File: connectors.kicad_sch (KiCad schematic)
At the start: 31 parts, among them J1 Conn_01x02, J2 USB_B_Micro, J3 Conn_01x04, J4 Conn_01x04, J5 Conn_01x04, J6 Conn_01x04, J7 Conn_01x04, J8 Conn_01x04, J9 Conn_02x05_Odd_Even, U4 USBLC6-2SC6

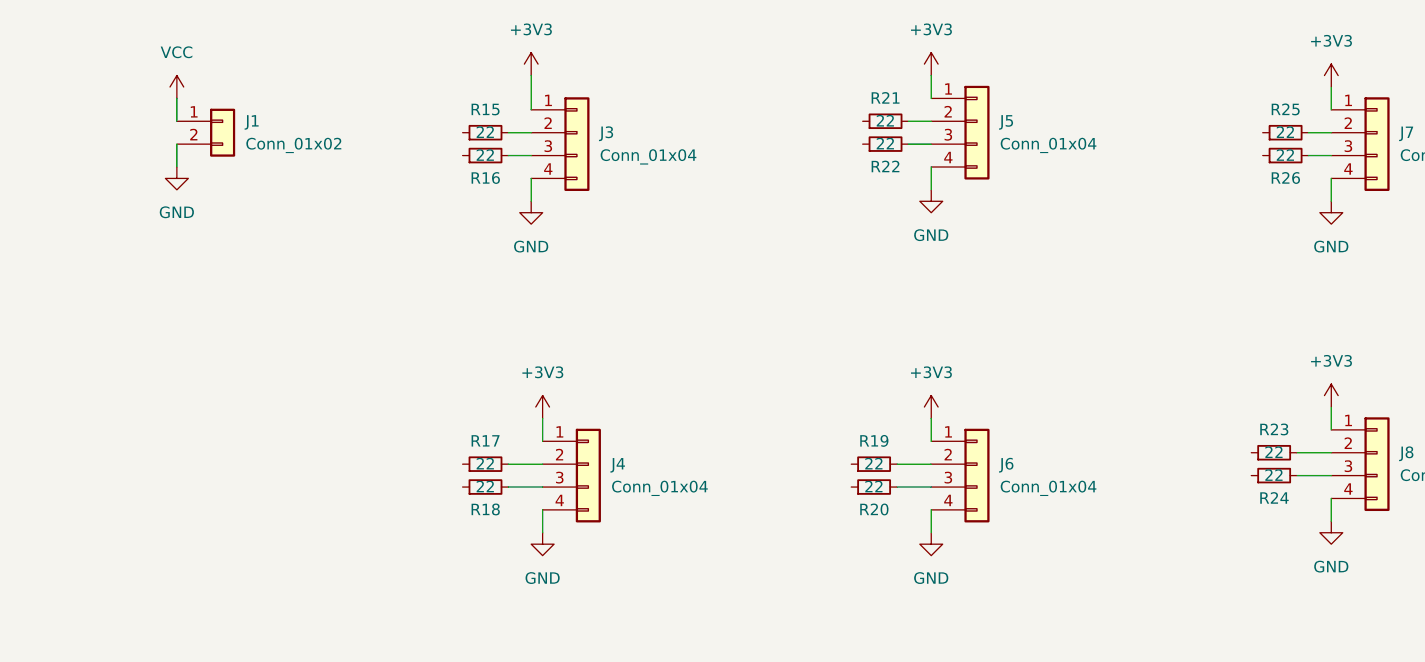
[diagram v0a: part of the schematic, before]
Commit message: updated schematic
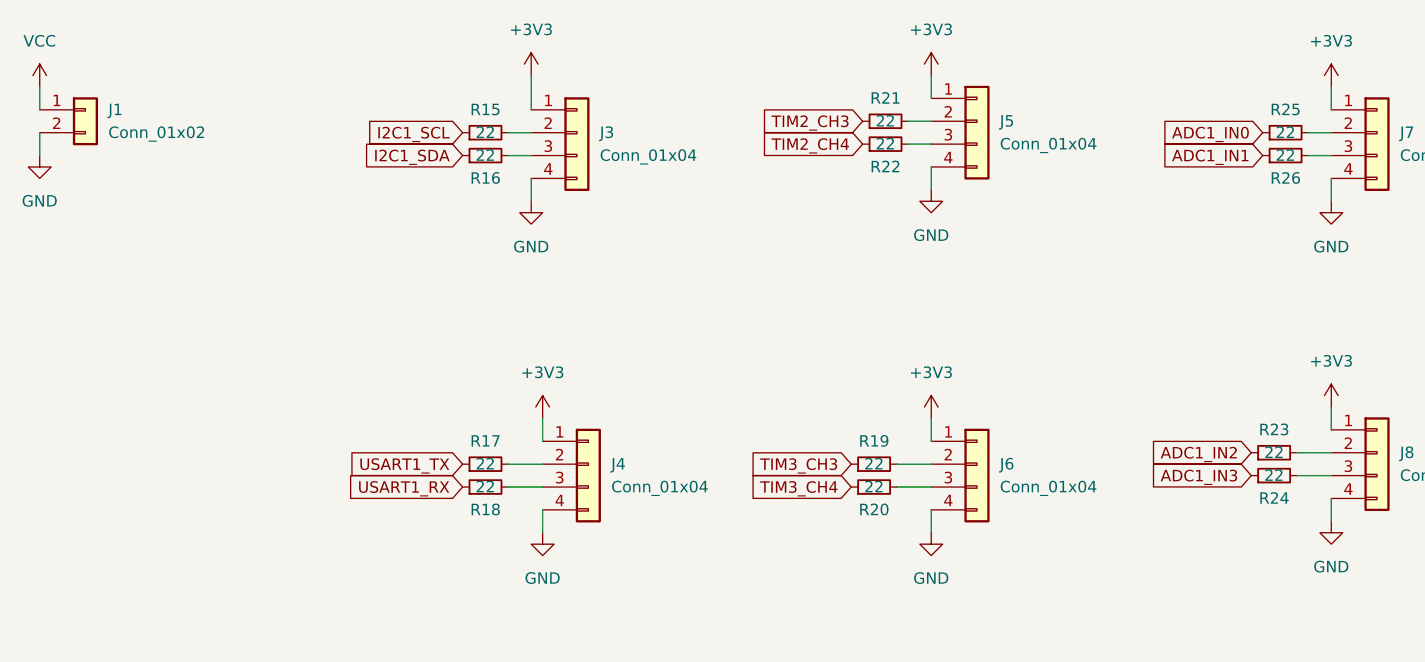
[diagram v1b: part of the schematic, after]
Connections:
- net TIM3_CH4: now reaches R20.1
- net USART1_RX: now reaches R18.1
- net TIM2_CH4: now reaches R22.1
- net USART1_TX: now reaches R17.1
- net I2C1_SCL: now reaches R15.1
- net ADC1_IN2: now reaches R23.1
- net ADC1_IN3: now reaches R24.1
- net ADC1_IN1: now reaches R26.1
- net TIM2_CH3: now reaches R21.1
- net TIM3_CH3: now reaches R19.1
- net ADC1_IN0: now reaches R25.1
- net I2C1_SDA: now reaches R16.1
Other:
- moved on the sheet: J1
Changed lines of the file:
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@@
     (stroke (width 0) (type default) (color 0 0 0 0))
   )
-  (wire (pts (xy 38.1 58.42) (xy 38.1 55.88))
+  (wire (pts (xy 22.86 57.15) (xy 22.86 54.61))
     (stroke (width 0) (type default) (color 0 0 0 0))
   )
@@
     (stroke (width 0) (type default) (color 0 0 0 0))
   )
-  (wire (pts (xy 38.1 50.8) (xy 38.1 53.34))
+  (wire (pts (xy 22.86 49.53) (xy 22.86 52.07))
     (stroke (width 0) (type default) (color 0 0 0 0))
   )
@@
     (stroke (width 0) (type default) (color 0 0 0 0))
   )
+  (global_label "I2C1_SCL" (shape input) (at 69.85 54.61 180) (fields_autoplaced)
+    (effects (font (size 1.27 1.27)) (justify right))
+    (property "Intersheet References" "${INTERSHEET_REFS}" (id 0) (at 58.6679 54.5306 0)
+      (effects (font (size 1.27 1.27)) (justify right) hide)
+    )
+  )
+  (global_label "I2C1_SDA" (shape input) (at 69.85 57.15 180) (fields_autoplaced)
+    (effects (font (size 1.27 1.27)) (justify right))
+    (property "Intersheet References" "${INTERSHEET_REFS}" (id 0) (at 58.6074 57.0706 0)
+      (effects (font (size 1.27 1.27)) (justify right) hide)
+    )
+  )
   (global_label "USB_D-" (shape input) (at 116.84 139.7 180) (fields_autoplaced)
     (effects (font (size 1.27 1.27)) (justify right))
     (property "Intersheet References" "${INTERSHEET_REFS}" (id 0) (at 106.8069 139.6206 0)
+      (effects (font (size 1.27 1.27)) (justify right) hide)
+    )
+  )
+  (global_label "ADC1_IN3" (shape input) (at 157.48 92.71 180) (fields_autoplaced)
+    (effects (font (size 1.27 1.27)) (justify right))
+    (property "Intersheet References" "${INTERSHEET_REFS}" (id 0) (at 146.1164 92.6306 0)
       (effects (font (size 1.27 1.27)) (justify right) hide)
     )
@@
     )
   )
+  (global_label "ADC1_IN2" (shape input) (at 157.48 90.17 180) (fields_autoplaced)
+    (effects (font (size 1.27 1.27)) (justify right))
+    (property "Intersheet References" "${INTERSHEET_REFS}" (id 0) (at 146.1164 90.0906 0)
+      (effects (font (size 1.27 1.27)) (justify right) hide)
+    )
+  )
+  (global_label "USART1_RX" (shape input) (at 69.85 93.98 180) (fields_autoplaced)
+    (effects (font (size 1.27 1.27)) (justify right))
+    (property "Intersheet References" "${INTERSHEET_REFS}" (id 0) (at 56.914 93.9006 0)
+      (effects (font (size 1.27 1.27)) (justify right) hide)
+    )
+  )
+  (global_label "TIM3_CH3" (shape input) (at 113.03 91.44 180) (fields_autoplaced)
+    (effects (font (size 1.27 1.27)) (justify right))
+    (property "Intersheet References" "${INTERSHEET_REFS}" (id 0) (at 101.6059 91.3606 0)
+      (effects (font (size 1.27 1.27)) (justify right) hide)
+    )
+  )
   (global_label "NRST" (shape input) (at 257.81 78.74 0) (fields_autoplaced)
     (effects (font (size 1.27 1.27)) (justify left))
@@
     )
   )
+  (global_label "ADC1_IN0" (shape input) (at 158.75 54.61 180) (fields_autoplaced)
+    (effects (font (size 1.27 1.27)) (justify right))
+    (property "Intersheet References" "${INTERSHEET_REFS}" (id 0) (at 147.3864 54.5306 0)
+      (effects (font (size 1.27 1.27)) (justify right) hide)
+    )
+  )
+  (global_label "USART1_TX" (shape input) (at 69.85 91.44 180) (fields_autoplaced)
+    (effects (font (size 1.27 1.27)) (justify right))
+    (property "Intersheet References" "${INTERSHEET_REFS}" (id 0) (at 57.2164 91.3606 0)
+      (effects (font (size 1.27 1.27)) (justify right) hide)
+    )
+  )
   (global_label "SWDIO" (shape input) (at 257.81 68.58 0) (fields_autoplaced)
     (effects (font (size 1.27 1.27)) (justify left))
@@
     )
   )
+  (global_label "TIM3_CH4" (shape input) (at 113.03 93.98 180) (fields_autoplaced)
+    (effects (font (size 1.27 1.27)) (justify right))
+    (property "Intersheet References" "${INTERSHEET_REFS}" (id 0) (at 101.6059 93.9006 0)
+      (effects (font (size 1.27 1.27)) (justify right) hide)
+    )
+  )
+  (global_label "ADC1_IN1" (shape input) (at 158.75 57.15 180) (fields_autoplaced)
+    (effects (font (size 1.27 1.27)) (justify right))
+    (property "Intersheet References" "${INTERSHEET_REFS}" (id 0) (at 147.3864 57.0706 0)
+      (effects (font (size 1.27 1.27)) (justify right) hide)
+    )
+  )
+  (global_label "TIM2_CH3" (shape input) (at 114.3 53.34 180) (fields_autoplaced)
+    (effects (font (size 1.27 1.27)) (justify right))
+    (property "Intersheet References" "${INTERSHEET_REFS}" (id 0) (at 102.8759 53.2606 0)
+      (effects (font (size 1.27 1.27)) (justify right) hide)
+    )
+  )
+  (global_label "TIM2_CH4" (shape input) (at 114.3 55.88 180) (fields_autoplaced)
+    (effects (font (size 1.27 1.27)) (justify right))
+    (property "Intersheet References" "${INTERSHEET_REFS}" (id 0) (at 102.8759 55.8006 0)
+      (effects (font (size 1.27 1.27)) (justify right) hide)
+    )
+  )
   (global_label "SWO" (shape input) (at 257.81 73.66 0) (fields_autoplaced)
     (effects (font (size 1.27 1.27)) (justify left))
@@
     (pin "1")
   )
-  (symbol (lib_id "power:VCC") (at 38.1 50.8 0) (unit 1)
-    (in_bom yes) (on_board yes) (fields_autoplaced)
-    (property "Reference" "#PWR030" (id 0) (at 38.1 54.61 0)
-      (effects (font (size 1.27 1.27)) hide)
-    )
-    (property "Value" "VCC" (id 1) (at 38.1 45.72 0))
-    (property "Footprint" "" (id 2) (at 38.1 50.8 0)
-      (effects (font (size 1.27 1.27)) hide)
-    )
-    (property "Datasheet" "" (id 3) (at 38.1 50.8 0)
+  (symbol (lib_id "power:VCC") (at 22.86 49.53 0) (unit 1)
+    (in_bom yes) (on_board yes) (fields_autoplaced)
+    (property "Reference" "#PWR030" (id 0) (at 22.86 53.34 0)
+      (effects (font (size 1.27 1.27)) hide)
+    )
+    (property "Value" "VCC" (id 1) (at 22.86 44.45 0))
+    (property "Footprint" "" (id 2) (at 22.86 49.53 0)
+      (effects (font (size 1.27 1.27)) hide)
+    )
+    (property "Datasheet" "" (id 3) (at 22.86 49.53 0)
       (effects (font (size 1.27 1.27)) hide)
     )
@@
     (pin "1")
   )
-  (symbol (lib_id "Connector_Generic:Conn_01x02") (at 43.18 53.34 0) (unit 1)
-    (in_bom yes) (on_board yes) (fields_autoplaced)
-    (property "Reference" "J1" (id 0) (at 45.72 53.3399 0)
-      (effects (font (size 1.27 1.27)) (justify left))
-    )
-    (property "Value" "Conn_01x02" (id 1) (at 45.72 55.8799 0)
-      (effects (font (size 1.27 1.27)) (justify left))
-    )
-    (property "Footprint" "" (id 2) (at 43.18 53.34 0)
-      (effects (font (size 1.27 1.27)) hide)
-    )
-    (property "Datasheet" "~" (id 3) (at 43.18 53.34 0)
+  (symbol (lib_id "Connector_Generic:Conn_01x02") (at 27.94 52.07 0) (unit 1)
+    (in_bom yes) (on_board yes) (fields_autoplaced)
+    (property "Reference" "J1" (id 0) (at 30.48 52.0699 0)
+      (effects (font (size 1.27 1.27)) (justify left))
+    )
+    (property "Value" "Conn_01x02" (id 1) (at 30.48 54.6099 0)
+      (effects (font (size 1.27 1.27)) (justify left))
+    )
+    (property "Footprint" "" (id 2) (at 27.94 52.07 0)
+      (effects (font (size 1.27 1.27)) hide)
+    )
+    (property "Datasheet" "~" (id 3) (at 27.94 52.07 0)
       (effects (font (size 1.27 1.27)) hide)
     )
@@
     (pin "1")
   )
-  (symbol (lib_id "power:GND") (at 38.1 58.42 0) (unit 1)
-    (in_bom yes) (on_board yes) (fields_autoplaced)
-    (property "Reference" "#PWR031" (id 0) (at 38.1 64.77 0)
-      (effects (font (size 1.27 1.27)) hide)
-    )
-    (property "Value" "GND" (id 1) (at 38.1 63.5 0))
-    (property "Footprint" "" (id 2) (at 38.1 58.42 0)
-      (effects (font (size 1.27 1.27)) hide)
-    )
-    (property "Datasheet" "" (id 3) (at 38.1 58.42 0)
-      (effects (font (size 1.27 1.27)) hide)
-    )
+  (symbol (lib_id "power:GND") (at 22.86 57.15 0) (unit 1)
+    (in_bom yes) (on_board yes) (fields_autoplaced)
+    (property "Reference" "#PWR031" (id 0) (at 22.86 63.5 0)
+      (effects (font (size 1.27 1.27)) hide)
+    )
+    (property "Value" "GND" (id 1) (at 22.86 62.23 0))
+    (property "Footprint" "" (id 2) (at 22.86 57.15 0)
+      (effects (font (size 1.27 1.27)) hide)
+    )
+    (property "Datasheet" "" (id 3) (at 22.86 57.15 0)
+      (effects (font (size 1.27 1.27)) hide)
+    )
